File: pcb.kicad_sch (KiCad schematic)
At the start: 1 part, among them J1 PTHF-126-02-GF-Q-368

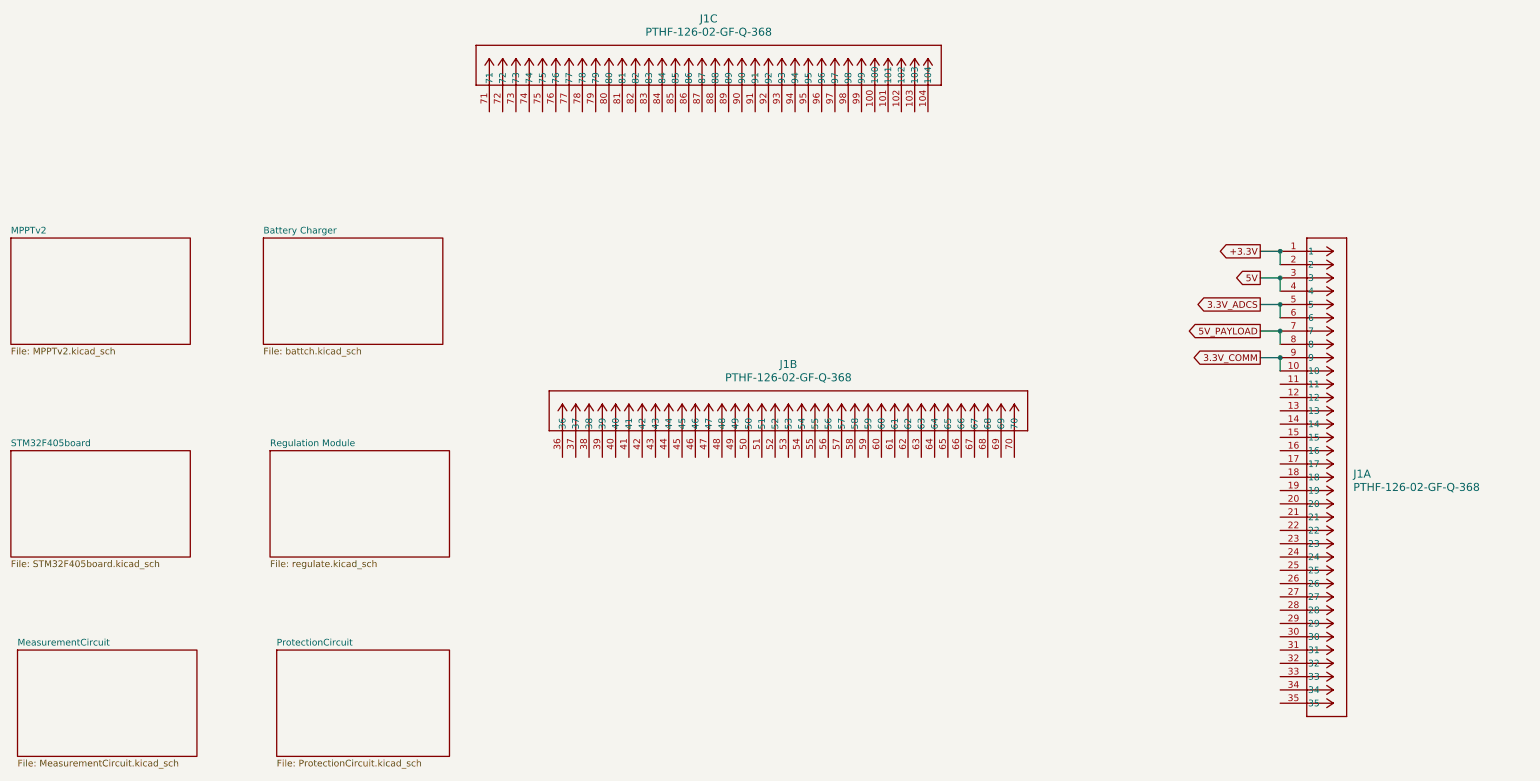
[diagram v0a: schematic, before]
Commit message: updates
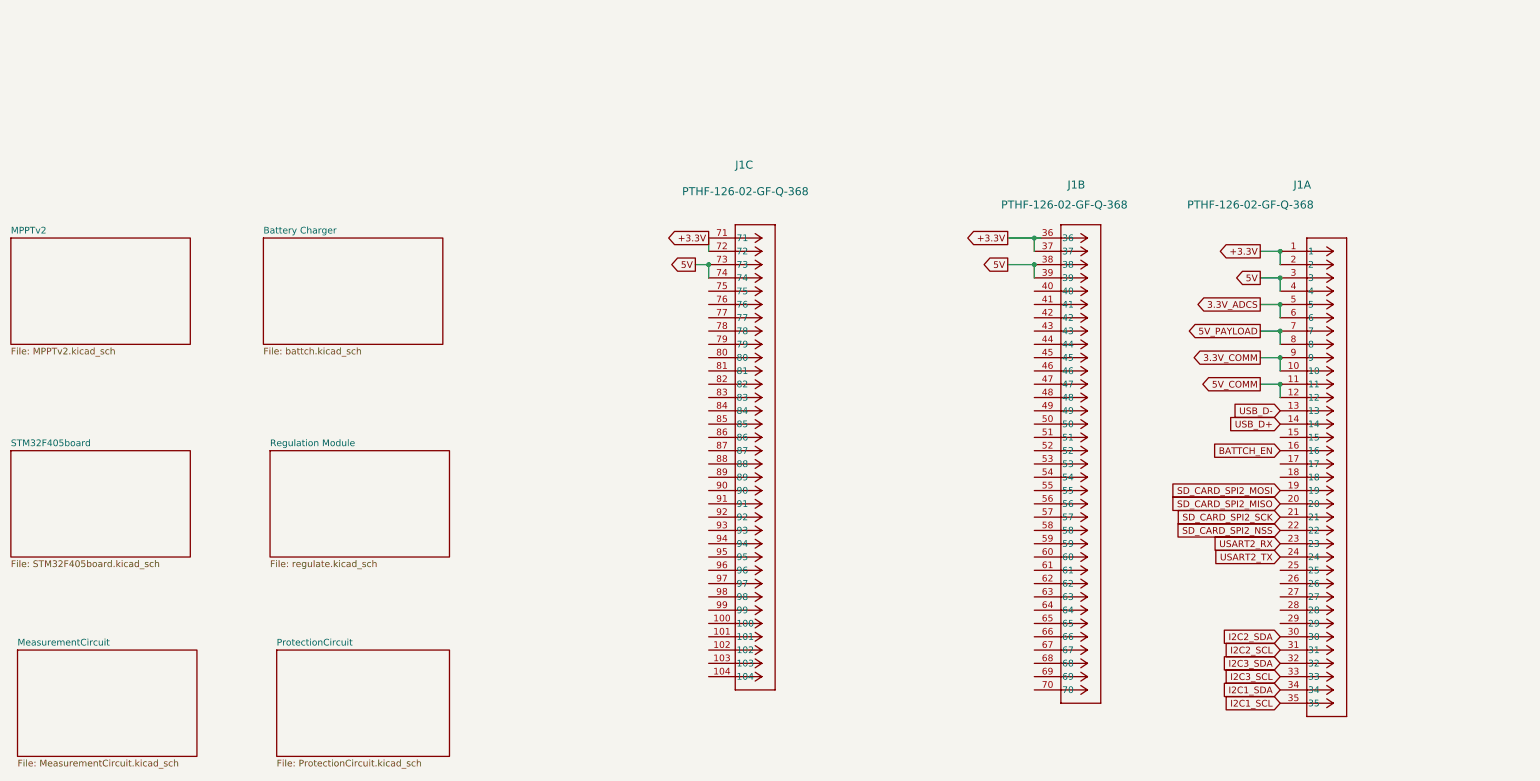
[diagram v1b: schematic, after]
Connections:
- net +3.3V: now also J1.36, J1.37, J1.71, J1.72
- net 5V: now also J1.38, J1.39, J1.73, J1.74
- net 5V_COMM: now reaches J1.11
- net 5V_COMM: now also J1.12
- net USB_D-: now reaches J1.13
- net USB_D+: now reaches J1.14
- net BATTCH_EN: now reaches J1.16
- net SD_CARD_SPI2_MOSI: now reaches J1.19
- net SD_CARD_SPI2_MISO: now reaches J1.20
- net SD_CARD_SPI2_SCK: now reaches J1.21
- net SD_CARD_SPI2_NSS: now reaches J1.22
- net USART2_RX: now reaches J1.23
- net USART2_TX: now reaches J1.24
- net I2C2_SDA: now reaches J1.30
- net I2C2_SCL: now reaches J1.31
- net I2C3_SDA: now reaches J1.32
- net I2C3_SCL: now reaches J1.33
- net I2C1_SDA: now reaches J1.34
- net I2C1_SCL: now reaches J1.35
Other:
- moved on the sheet: J1B, J1C
